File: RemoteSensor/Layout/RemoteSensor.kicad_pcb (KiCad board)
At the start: 2 copper layers, 50.8 x 50.8 mm, 47 parts, among them J1 PRG_HEADER, J2 LCD_HEADER, J3 USB_B_Micro, J4 BATT_CONN, Q1 2N7002, Q2 2N7002, Q3 2N7002, SW1 BTN_RST, SW2 BTN_LOAD, SW3 SW_DPDT_x2, U1 ESP-12F, U2 74LVC2G02, U3 LM50CIM3, U4 MCP73831-2-OT, U5 LM3670MF, U6 BD48ExxG, U7 BD48ExxG

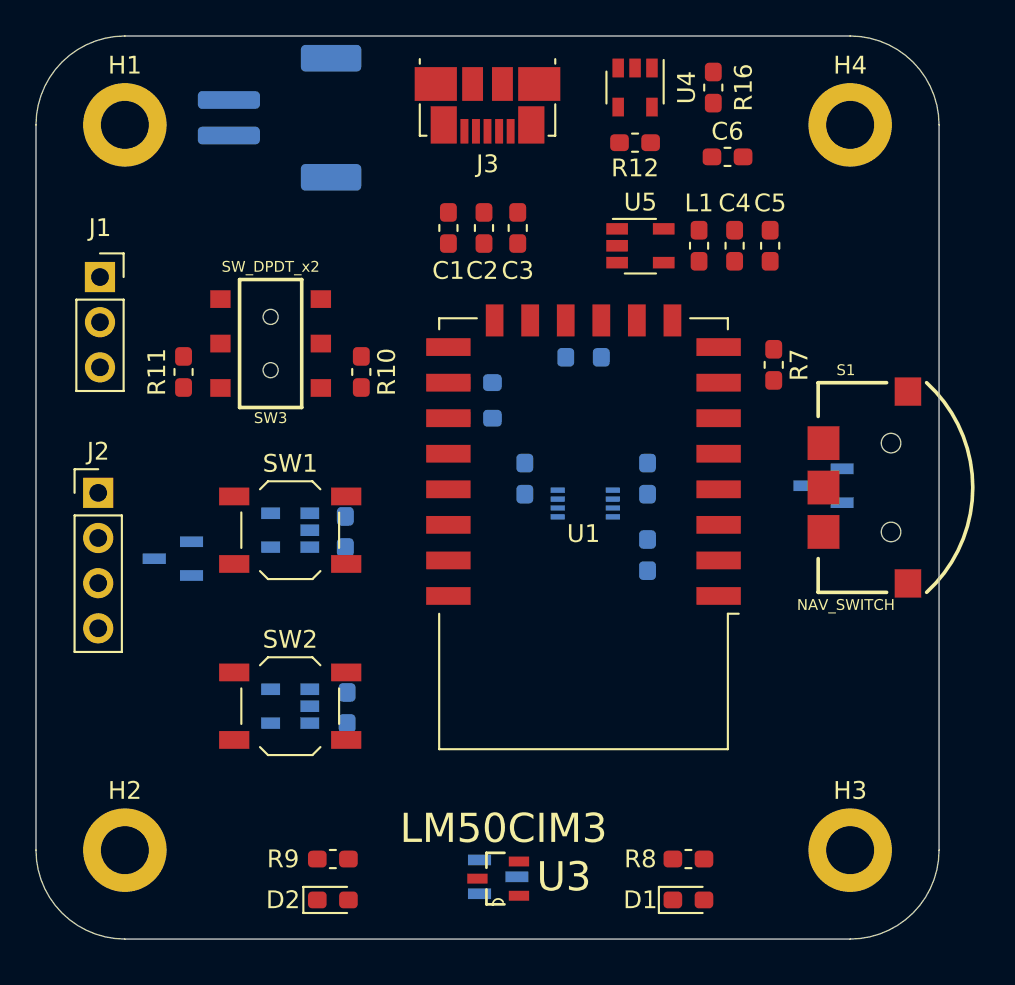
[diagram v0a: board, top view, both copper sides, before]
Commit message: Edit layout
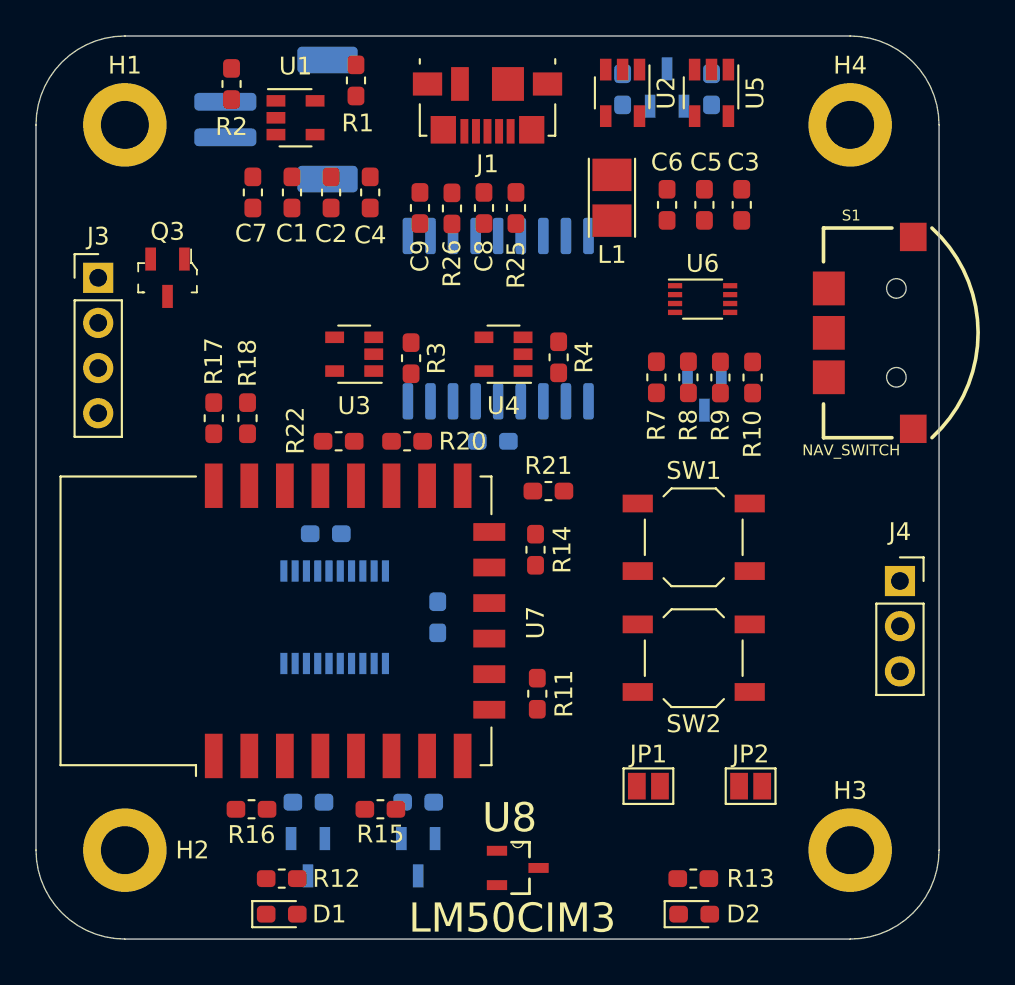
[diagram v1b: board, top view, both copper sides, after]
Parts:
- removed SW3: SW_DPDT_x2, Switches:SWITCH_DPDT_SMD_AYZ0202
- added C10: 100n, Capacitor_SMD:C_0603_1608Metric_Pad1.05x0.95mm_HandSolder, B.Cu at (130.6, 92.3)
- added C7: 4.7u, Capacitor_SMD:C_0603_1608Metric_Pad1.05x0.95mm_HandSolder, F.Cu at (126.5, 73.1)
- added C8: 47p, Capacitor_SMD:C_0603_1608Metric_Pad1.05x0.95mm_HandSolder, F.Cu at (139.5, 74.0)
- added C9: 47p, Capacitor_SMD:C_0603_1608Metric_Pad1.05x0.95mm_HandSolder, F.Cu at (135.9, 74.0)
- added FB1: Ferrite_Bead, Resistor_SMD:R_0603_1608Metric_Pad1.05x0.95mm_HandSolder, B.Cu at (136.9, 97.0)
- added JP1: Jumper_2_Open, Jumper:SolderJumper-2_P1.3mm_Open_Pad1.0x1.5mm, F.Cu at (148.8, 106.5)
- added JP2: Jumper_2_Open, Jumper:SolderJumper-2_P1.3mm_Open_Pad1.0x1.5mm, F.Cu at (154.5, 106.5)
- added Q4: MMBT2222A-TP, digikey-footprints:SOT-23-3, B.Cu at (129.6, 110.5)
- added Q5: MMBT2222A-TP, digikey-footprints:SOT-23-3, B.Cu at (135.8, 110.5)
- added R17: 1k, Resistor_SMD:R_0603_1608Metric_Pad1.05x0.95mm_HandSolder, F.Cu at (124.3, 85.8)
- added R18: 1k, Resistor_SMD:R_0603_1608Metric_Pad1.05x0.95mm_HandSolder, F.Cu at (126.2, 85.8)
- added R19: 10k, Resistor_SMD:R_0603_1608Metric_Pad1.05x0.95mm_HandSolder, B.Cu at (140.0, 87.1)
- added R20: 10k, Resistor_SMD:R_0603_1608Metric_Pad1.05x0.95mm_HandSolder, F.Cu at (135.2, 87.1)
- added R21: 10k, Resistor_SMD:R_0603_1608Metric_Pad1.05x0.95mm_HandSolder, F.Cu at (143.1, 89.9)
- added R22: 10k, Resistor_SMD:R_0603_1608Metric_Pad1.05x0.95mm_HandSolder, F.Cu at (131.3, 87.1)
- added R23: 10k, Resistor_SMD:R_0603_1608Metric_Pad1.05x0.95mm_HandSolder, B.Cu at (135.8, 107.4)
- added R24: 10k, Resistor_SMD:R_0603_1608Metric_Pad1.05x0.95mm_HandSolder, B.Cu at (129.6, 107.4)
- added R25: 27, Resistor_SMD:R_0603_1608Metric_Pad1.05x0.95mm_HandSolder, F.Cu at (141.3, 74.0)
- added R26: 27, Resistor_SMD:R_0603_1608Metric_Pad1.05x0.95mm_HandSolder, F.Cu at (137.7, 74.0)
- added U10: FT231XS, Package_SO:SSOP-20_3.9x8.7mm_P0.635mm, B.Cu at (131.1, 97.0)
- added U8: LM50CIM3, LM50CIM3:SOT95P260X110-3N, F.Cu at (141.4, 111.1)
- added U9: MCP23008-E_P, Package_SO:SOIC-18W_7.5x11.6mm_P1.27mm, B.Cu at (140.3, 80.2)
- C3: value 4.7u -> 10u
- C4: value 10u -> 4.7u
- J1: value PRG_HEADER -> USB_B_Micro; footprint Connector_PinSocket_2.54mm:PinSocket_1x03_P2.54mm_Vertical -> Connector_USB:USB_Micro-B_Molex_47346-0001
- J2: value LCD_HEADER -> BATT_CONN; footprint Connector_PinHeader_2.54mm:PinHeader_1x04_P2.54mm_Vertical -> Connector_JST:JST_PH_S2B-PH-SM4-TB_1x02-1MP_P2.00mm_Horizontal; moved to B.Cu
- J3: value USB_B_Micro -> LCD_HEADER; footprint Connector_USB:USB_Micro-B_Molex_47346-0001 -> Connector_PinHeader_2.54mm:PinHeader_1x04_P2.54mm_Vertical
- J4: value BATT_CONN -> PRG_HEADER; footprint Connector_JST:JST_PH_S2B-PH-SM4-TB_1x02-1MP_P2.00mm_Horizontal -> Connector_PinSocket_2.54mm:PinSocket_1x03_P2.54mm_Vertical; moved to F.Cu
- L1: footprint Inductor_SMD:L_0603_1608Metric_Pad1.05x0.95mm_HandSolder -> Inductor_SMD:L_Taiyo-Yuden_NR-24xx_HandSoldering
- Q3, R15, R2, R3, R4: moved to F.Cu
- R1: value 10k -> 2k; moved to F.Cu
- R10: value 1k -> 10k
- R11: value 1k -> 4.7k
- R12: value 2k -> 100
- R13: value 10k -> 100; moved to F.Cu
- R14: value 10k -> 4.7k; moved to F.Cu
- R5, R6: value 4.7k -> 10k
- R8, R9: value 220 -> 10k
- SW2: value BTN_LOAD -> SW_Push
- U1: value ESP-12F -> MCP73831-2-OT; footprint RF_Module:ESP-12E -> Package_TO_SOT_SMD:SOT-23-5
- U2: value 74LVC2G02 -> LM3671MF; footprint Package_SO:VSSOP-8_2.3x2mm_P0.5mm -> Package_TO_SOT_SMD:TSOT-23-5; moved to F.Cu
- U3: value LM50CIM3 -> BD48ExxG; footprint LM50CIM3:SOT95P260X110-3N -> Package_TO_SOT_SMD:SOT-23-5
- U4: value MCP73831-2-OT -> BD48ExxG
- U5: value LM3670MF -> LM3671MF
- U6: value BD48ExxG -> 74LVC2G02; footprint Package_TO_SOT_SMD:SOT-23-5 -> Package_SO:VSSOP-8_2.3x2mm_P0.5mm; moved to F.Cu
- U7: value BD48ExxG -> ESP-12F; footprint Package_TO_SOT_SMD:SOT-23-5 -> RF_Module:ESP-12E; moved to F.Cu
- moved R16 48.2 mm to (126.4, 107.8), turned to 180 degrees
- moved R12 45.9 mm to (128.1, 111.7), turned to 0 degrees
- moved J4 43.6 mm to (162.9, 95.0), turned to 0 degrees
- moved R9 34.8 mm to (152.8, 83.5), turned to 270 degrees
- moved U6 32.6 mm to (151.8, 79.1), turned to 0 degrees
- moved R1 31.3 mm to (132.3, 66.8)
- moved U3 30.6 mm to (132.2, 82.2)
- moved Q2 29.7 mm to (151.9, 84.3), turned to 270 degrees
- moved U1 28.5 mm to (128.9, 68.9), turned to 0 degrees
- moved R8 27.1 mm to (151.0, 83.5), turned to 270 degrees
- moved R11 26.9 mm to (142.5, 101.3), turned to 90 degrees
- moved R13 24.4 mm to (151.3, 111.7), turned to 180 degrees
- moved Q1 24.1 mm to (149.8, 67.2), turned to 90 degrees
- moved J3 24.0 mm to (117.8, 77.9), turned to 0 degrees
- moved J1 23.8 mm to (139.7, 68.2), turned to 180 degrees
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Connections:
- C3 pad 1: V_BATT -> 3.3V
- C4 pad 1: 3.3V -> V_USB
- J1 pad 1: Net-(J1-Pad1) -> V_USB
- J1 pad 2: GND -> USBDM
- J1 pad 3: Net-(J1-Pad3) -> USBDP
- J2 pad 1: 3.3V -> V_BATT
- J2 pad 2: Net-(J2-Pad2) -> GND
- J3 pad 1: V_USB -> 3.3V
- J3 pad 2: (no net) -> Net-(J3-Pad2)
- J3 pad 3: (no net) -> /Processor/SCL
- J3 pad 4: (no net) -> /Processor/SDA
- J4 pad 1: GND -> PRG_TX
- J4 pad 2: V_BATT -> GND
- L1 pad 1: Net-(L1-Pad1) -> /Power/SW
- Q1 pad 1: /SLEEP_STS -> V_USB
- Q1 pad 2: /CENTER_PIN -> GND
- Q1 pad 3: /RST -> Net-(Q1-Pad3)
- Q2 pad 1: /WAKE_STS -> SLEEP_STS
- Q2 pad 2: GND -> CENTER_BTN
- Q2 pad 3: Net-(Q2-Pad3) -> RST
- Q3 pad 1: /WAKE_STS -> WAKE_STS
- Q3 pad 3: Net-(J2-Pad2) -> Net-(J3-Pad2)
- R1 pad 1: 3.3V -> Net-(R1-Pad1)
- R1 pad 2: /RST -> GND
- R10 pad 1: Net-(J1-Pad1) -> SLEEP_STS
- R10 pad 2: /PRG_TX -> GND
- R11 pad 1: Net-(J1-Pad3) -> 3.3V
- R11 pad 2: /PRG_RX -> /Processor/SCL
- R12 pad 1: Net-(R12-Pad1) -> HB_PIN
- R12 pad 2: GND -> Net-(D1-Pad2)
- R13 pad 1: /WAKE_STS -> Net-(D2-Pad2)
- R13 pad 2: GND -> BATT_PIN
- R14 pad 2: /CHARGER_STS -> /Processor/SDA
- R15 pad 2: /BATT_STS -> Net-(R15-Pad2)
- R16 pad 2: /CHARGE_STS -> RST
- R2 pad 1: /SLEEP_PIN -> 3.3V
- R2 pad 2: GND -> CHARGE_STS
- R3 pad 1: /HB_PIN -> 3.3V
- R3 pad 2: GND -> BATT_STS
- R4 pad 1: /SLEEP_STS -> 3.3V
- R4 pad 2: GND -> CHARGER_STS
- R5 pad 1: 3.3V -> V_USB
- R5 pad 2: /SCL -> GND
- R6 pad 1: 3.3V -> V_BATT
- R6 pad 2: /SDA -> Net-(Q1-Pad3)
- R7 pad 1: 3.3V -> SLEEP_PIN
- R7 pad 2: Net-(R7-Pad2) -> GND
- R8 pad 1: /HB_PIN -> WAKE_STS
- R8 pad 2: Net-(D1-Pad2) -> GND
- R9 pad 1: Net-(D2-Pad2) -> HB_PIN
- R9 pad 2: /BATT_PIN -> GND
- S1 pad 1: /UP_PIN -> UP_BTN
- S1 pad 2: /DOWN_PIN -> DOWN_BTN
- S1 pad T: /CENTER_PIN -> CENTER_BTN
- SW1 pad 1: /RST -> RST
- SW2 pad 1: Net-(SW2-Pad1) -> FLASH
- U1 pad 1: /RST -> CHARGE_STS
- U1 pad 2: /TEMP_PIN -> GND
- U1 pad 3: Net-(R7-Pad2) -> V_BATT
- U1 pad 4: /RST -> V_USB
- U1 pad 5: /BATT_STS -> Net-(R1-Pad1)
- U2 pad 1: /SLEEP_PIN -> V_USB
- U2 pad 2: /SLEEP_STS -> GND
- U2 pad 3: /SLEEP_STS -> V_USB
- U2 pad 4: GND -> 3.3V
- U2 pad 5: /WAKE_STS -> /Power/SW
- U3 pad 1: 3.3V -> BATT_STS
- U3 pad 2: /TEMP_PIN -> V_BATT
- U3 pad 3: Net-(Q2-Pad3) -> GND
- U4 pad 1: /CHARGE_STS -> CHARGER_STS
- U4 pad 2: GND -> V_USB
- U4 pad 3: V_BATT -> GND
- U4 pad 4: V_USB -> (no net)
- U4 pad 5: Net-(R12-Pad1) -> (no net)
- U5 pad 3: V_BATT -> Net-(Q1-Pad3)
- U5 pad 5: Net-(L1-Pad1) -> /Power/SW
- U6 pad 1: /CHARGER_STS -> SLEEP_PIN
- U6 pad 2: 3.3V -> SLEEP_STS
- U6 pad 3: GND -> SLEEP_STS
- U6 pad 4: (no net) -> GND
- U6 pad 5: (no net) -> WAKE_STS
- U7 pad 1: /BATT_STS -> RST
- U7 pad 2: 3.3V -> /Processor/TEMP_PIN
- U7 pad 3: GND -> Net-(R15-Pad2)
- U7 pad 4: (no net) -> RST
